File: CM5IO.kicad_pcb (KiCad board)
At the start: 4 copper layers, 160 x 90 mm, 76 parts, among them J10 690-019-298-412, J11 USB_C_Receptacle_USB2.0, J12 USB3_A, J14 JST_SHBM04B-SRSS-TB, J16 Conn_01x22_Female, J2 Conn_02x07_Odd_Even, J22 690-019-298-412, J3 Conn_01x03, J4 Bus_M.2_Socket_M, J5 Conn_01x22_Female, J6 THD-02-R, J7 Micro_SD_Card_Det, J8 THD-20-R, J9 THD-02-R, SW1 Right angle Tact button, U1 TPD4EUSB30, U12 RT9742SNGV, U18 RT9742GGJ5, U2 TPD4EUSB30, U3 MagJack-A70-112-331N126, U5 74LVC1G07SE-7, U6 AP22653W6, U7 ASEK-32.768KHZ-L-R-T, U8 AP3441SHE-7B

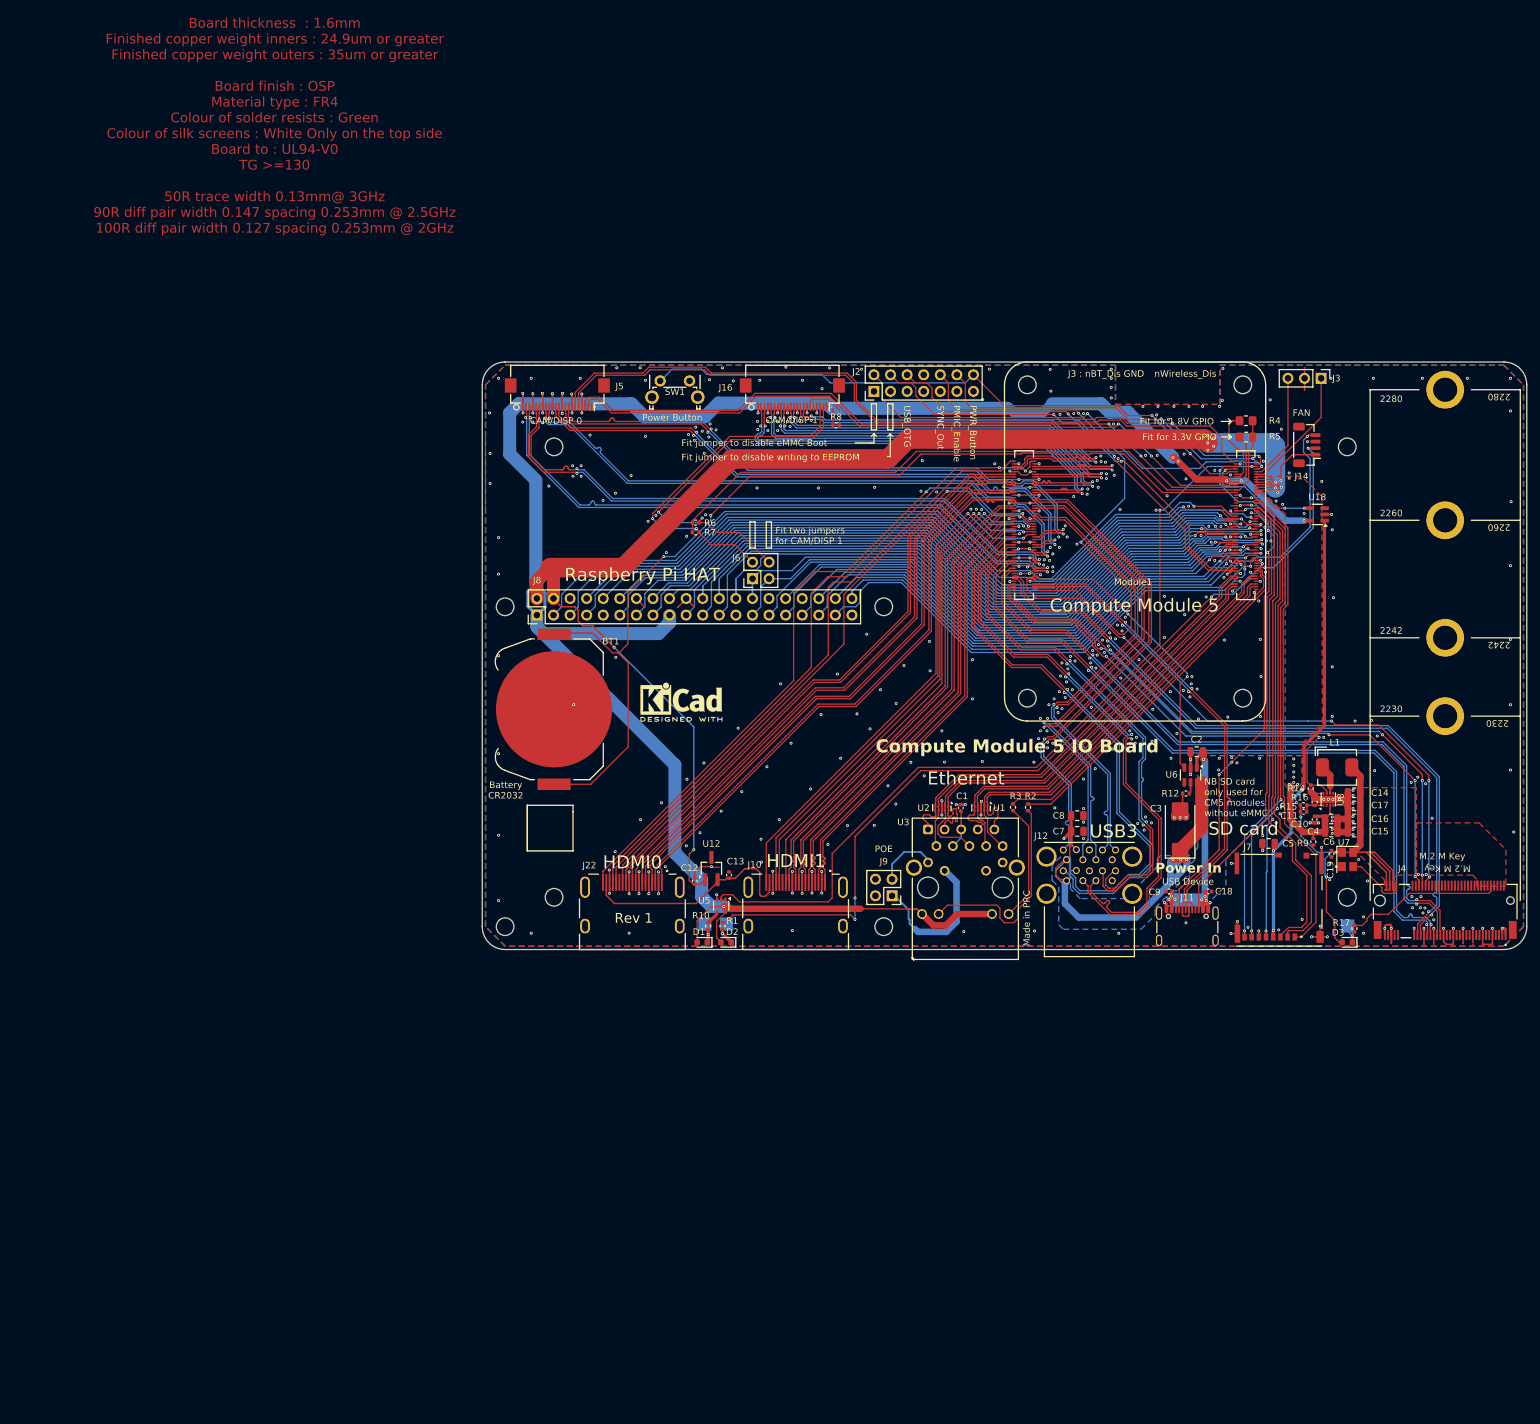
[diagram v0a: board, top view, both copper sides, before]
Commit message: first pass at layout
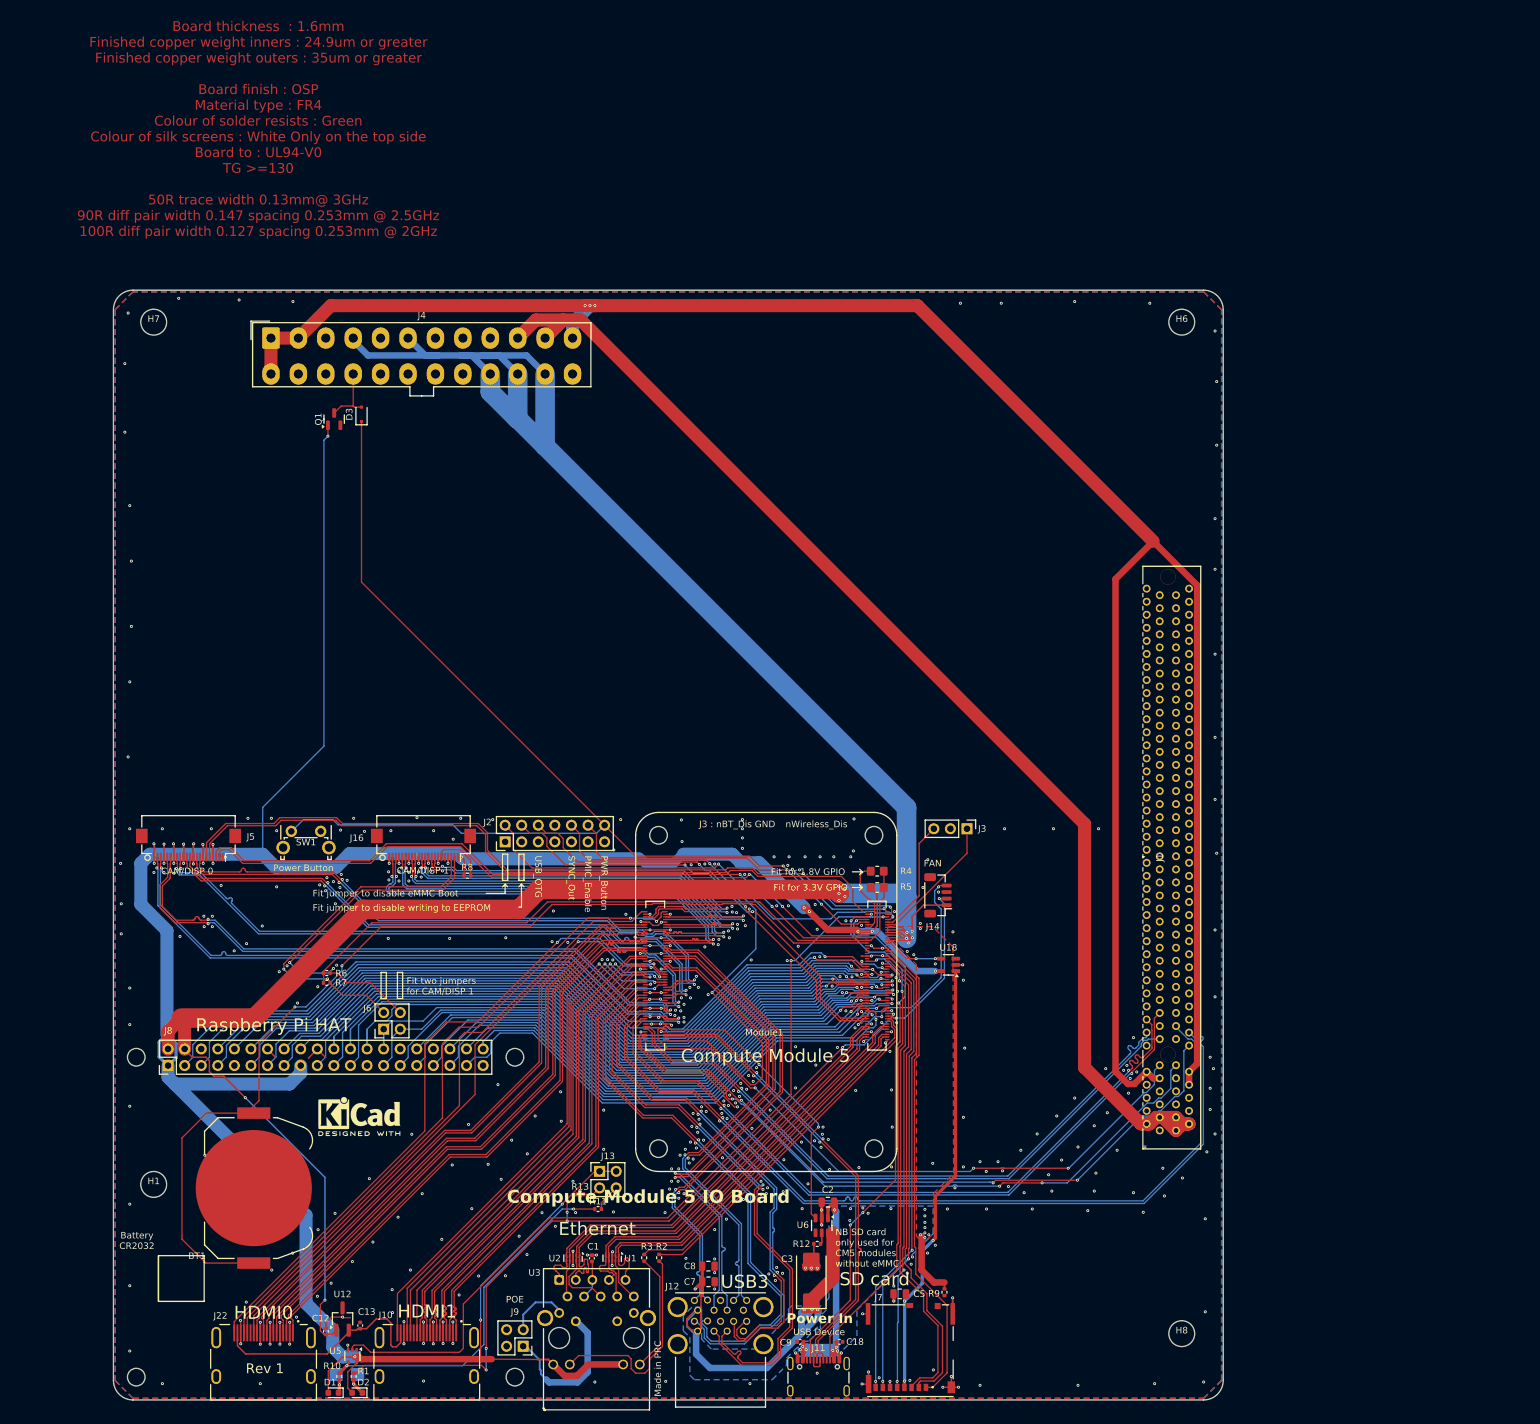
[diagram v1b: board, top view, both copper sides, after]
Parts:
- removed C10, C19: 100n, Capacitor_SMD:C_0402_1005Metric
- removed C11: 4.7nF, Capacitor_SMD:C_0402_1005Metric
- removed C14, C15, C16, C17, C4, C6: 10u, Capacitor_SMD:C_0805_2012Metric
- removed L1: 2.2uH, CM5IO:L_Bourns_SRP5030CC
- removed R14: 100K 1%, Resistor_SMD:R_0402_1005Metric
- removed R15: 10K 1%, Resistor_SMD:R_0402_1005Metric
- removed R16: 2.2K 1%, Resistor_SMD:R_0402_1005Metric
- removed R17: 1k, Resistor_SMD:R_0402_1005Metric
- removed TP1: TestPoint, TestPoint:TestPoint_Pad_2.0x2.0mm
- removed U7: ASEK-32.768KHZ-L-R-T, Crystal:Crystal_SMD_3225-4Pin_3.2x2.5mm
- removed U8: AP3441SHE-7B, Package_DFN_QFN:DFN-8-1EP_2x2mm_P0.5mm_EP1.05x1.75mm
- added J1: PCIE-164-02-F-D-TH, CM5IO:CONN_PCIE-164-02-x-D-TH_SAI, F.Cu at (182.8, 187.7)
- added J13: THD-02-R, Connector_PinHeader_2.54mm:PinHeader_2x02_P2.54mm_Vertical, F.Cu at (97.0, 194.0)
- added Q1: BS170F, Package_TO_SOT_SMD:SOT-23, F.Cu at (56.3, 78.8)
- added R11: 1k, Resistor_SMD:R_0402_1005Metric, F.Cu at (96.7, 199.8)
- added R13: 1k, Resistor_SMD:R_0402_1005Metric, F.Cu at (94.0, 197.5)
- D3: value LED Green -> D; footprint LED_SMD:LED_0603_1608Metric -> Diode_SMD:D_SOD-323F
- H1, H6, H7, H8: footprint CM5IO:MountingHole_2.7mm_M2.5_DIN965 -> CM5IO:atx_mountinghole
- J4: value Bus_M.2_Socket_M -> ATX-24; footprint CM5IO:M.2 M Key socket -> Connector_Molex:Molex_Mini-Fit_Jr_5566-24A_2x12_P4.20mm_Vertical
- moved J4 199.4 mm to (46.6, 66.3), turned to 0 degrees
- moved D3 171.3 mm to (60.5, 78.0), turned to 90 degrees
- moved J8 89.2 mm to (30.9, 177.8)
- moved C1 89.2 mm to (95.8, 207.3)
- moved J9 89.2 mm to (85.3, 220.8)
- moved R3 89.2 mm to (103.8, 207.2)
- moved TP3 89.2 mm to (59.9, 225.1)
- moved C12 89.2 mm to (55.0, 218.5)
- moved C13 89.2 mm to (60.3, 217.6)
- moved C18 89.2 mm to (133.7, 220.1)
- moved C2 89.2 mm to (131.9, 198.7)
- moved C3 89.2 mm to (129.4, 210.6)
- moved C5 89.2 mm to (142.9, 212.8)
- moved C7 89.2 mm to (113.7, 210.9)
- moved C8 89.2 mm to (113.6, 208.5)
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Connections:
- net Net-(Module1A-LED_nACT) renamed /CM5_GPIO ( Ethernet, GPIO, SDCARD)/LED_nACT
- D3 pad 1: Net-(D3-K) -> /PWR_BUT
- D3 pad 2: /PCIe-M2/M2_3v3 -> Net-(D3-A)
- J2 pad 14: /CM5_GPIO ( Ethernet, GPIO, SDCARD)/PWR_BUT -> /PWR_BUT
- J4 pad 1: GND -> /+3.3v_pcie
- J4 pad 10: Net-(J4-DAS/~{DSS}/~{LED1}) -> /+12v
- J4 pad 11: unconnected-(J4-PERn3-Pad11) -> /+12v
- J4 pad 12: /PCIe-M2/M2_3v3 -> /+3.3v_pcie
- J4 pad 13: unconnected-(J4-PERp3-Pad13) -> /+3.3v_pcie
- J4 pad 14: /PCIe-M2/M2_3v3 -> unconnected-(J4--12V-Pad14)
- J4 pad 16: /PCIe-M2/M2_3v3 -> Net-(D3-A)
- J4 pad 17: unconnected-(J4-PETn2-Pad17) -> GND
- J4 pad 18: /PCIe-M2/M2_3v3 -> GND
- J4 pad 19: unconnected-(J4-PETp2-Pad19) -> GND
- J4 pad 2: /PCIe-M2/M2_3v3 -> /+3.3v_pcie
- J4 pad 21: GND -> /+5v
- J4 pad 22: unconnected-(J4-NC-Pad22) -> /+5v
- J4 pad 23: unconnected-(J4-PERn2-Pad23) -> /+5v
- J4 pad 24: unconnected-(J4-NC-Pad24) -> GND
- J4 pad 4: /PCIe-M2/M2_3v3 -> /+5v
- J4 pad 5: unconnected-(J4-PETn3-Pad5) -> GND
- J4 pad 6: unconnected-(J4-NC-Pad6) -> /+5v
- J4 pad 7: unconnected-(J4-PETp3-Pad7) -> GND
- J4 pad 9: GND -> unconnected-(J4-+5VSB-Pad9)
- Module1 pad 106: /CM5_HighSpeed/PCIE_PWR_EN -> unconnected-(Module1B-PCIE_PWR_EN-Pad106)
- Module1 pad 92: /CM5_GPIO ( Ethernet, GPIO, SDCARD)/PWR_BUT -> /PWR_BUT
- SW1 pad 1: /CM5_GPIO ( Ethernet, GPIO, SDCARD)/PWR_BUT -> /PWR_BUT
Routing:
- net /+3.3v_pcie: track 0.00 -> 342.6 mm, vias 0 -> 3
- net /+12v: track 0.00 -> 187.4 mm
- net /PWR_BUT: track 0.00 -> 174.0 mm, vias 0 -> 2
- net /+5v: track 284.2 -> 450.5 mm
- net /+3.3v: track 324.6 -> 433.7 mm, vias 8 -> 11
- net /CM5_GPIO ( Ethernet, GPIO, SDCARD)/PWR_BUT: track 96.7 -> 0.00 mm, vias 2 -> 0
- net /CM5_HighSpeed/PCIE_PWR_EN: track 71.3 -> 0.00 mm, vias 2 -> 0
- net /PCIe-M2/M2_3v3: track 70.4 -> 0.00 mm, vias 3 -> 0
- net GND: track 766.8 -> 701.2 mm, vias 477 -> 487
- net Net-(R10-Pad2): track 2.22 -> 55.3 mm, vias 0 -> 2
- net Net-(J4-DAS/~{DSS}/~{LED1}): track 24.1 -> 0.00 mm
- net unconnected-(Module1B-PCIE_PWR_EN-Pad106): track 0.00 -> 22.1 mm, vias 0 -> 1
- net /CM5_HighSpeed/PCIE_TX_N: track 109.5 -> 130.3 mm, vias 2 -> 1
- net /CM5_HighSpeed/PCIE_TX_P: track 109.5 -> 130.1 mm, vias 2 -> 1
- net /CM5_HighSpeed/PCIE_nCLKREQ: track 92.1 -> 105.5 mm, vias 4 -> 3
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- removed copper zone on F.Cu, net /PCIe-M2/M2_3v3
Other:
- board size 160 x 90 mm -> 170 x 170 mm
- board text added: "+pwr -pwr"
- board text added: "act+ act-"
- board text removed: "M.2 M Key"
